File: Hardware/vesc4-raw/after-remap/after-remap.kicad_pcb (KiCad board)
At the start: 4 copper layers, 40.3 x 65 mm, 127 parts, among them K1 SERVO, P1 HALL/Encoder, P101 CANBUS, P2 SWD, P3 PWR_COMM, P4 IN+, P5 IN-, P6 MOTOR1, P7 MOTOR2, P9 MOTOR3, Q1 IPT007N06NATMA1, Q2 IPT007N06NATMA1, Q3 IPT007N06NATMA1, Q4 IPT007N06NATMA1, Q5 IPT007N06NATMA1, Q6 IPT007N06NATMA1, U1 STM32F40X_LQFP64, U2 TC2117, U3 DRV8302, U401 SN65HVD232, X2 8MHz 10ppm

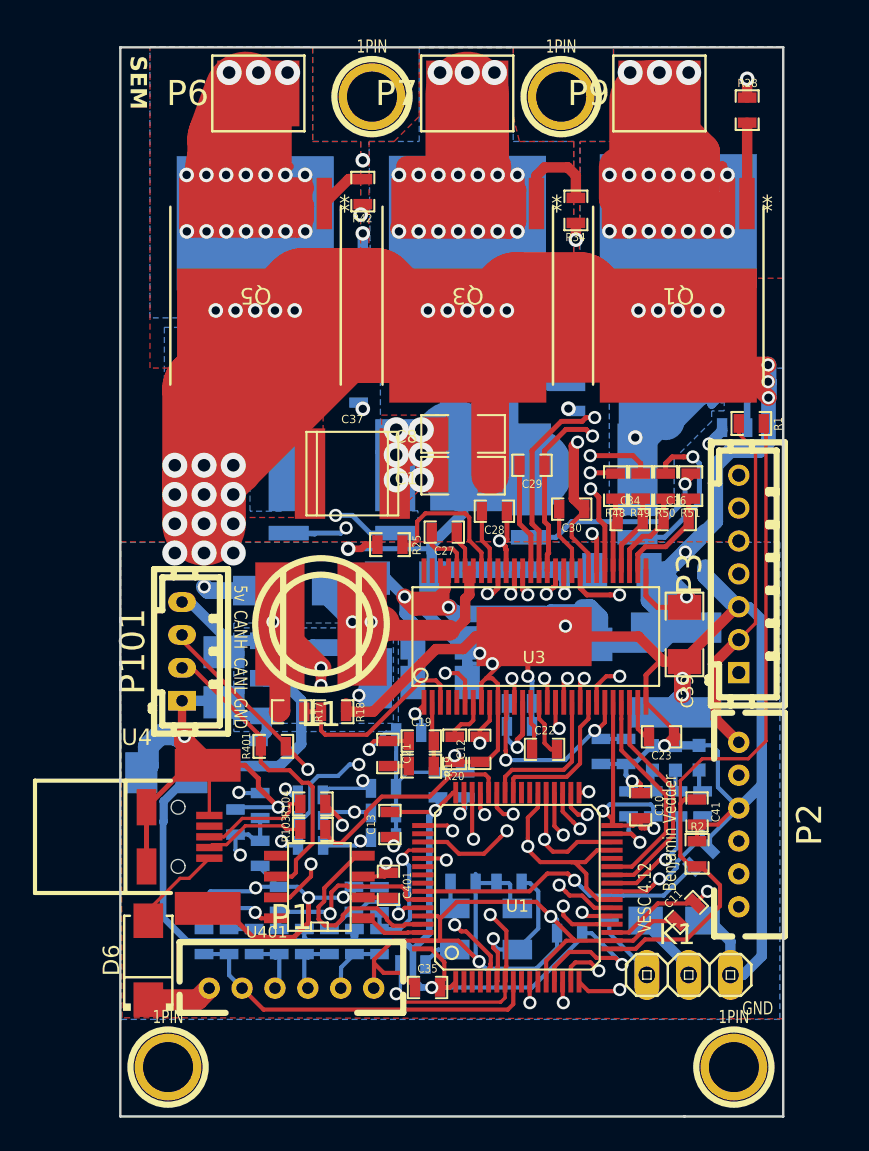
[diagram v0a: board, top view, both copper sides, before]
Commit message: cp
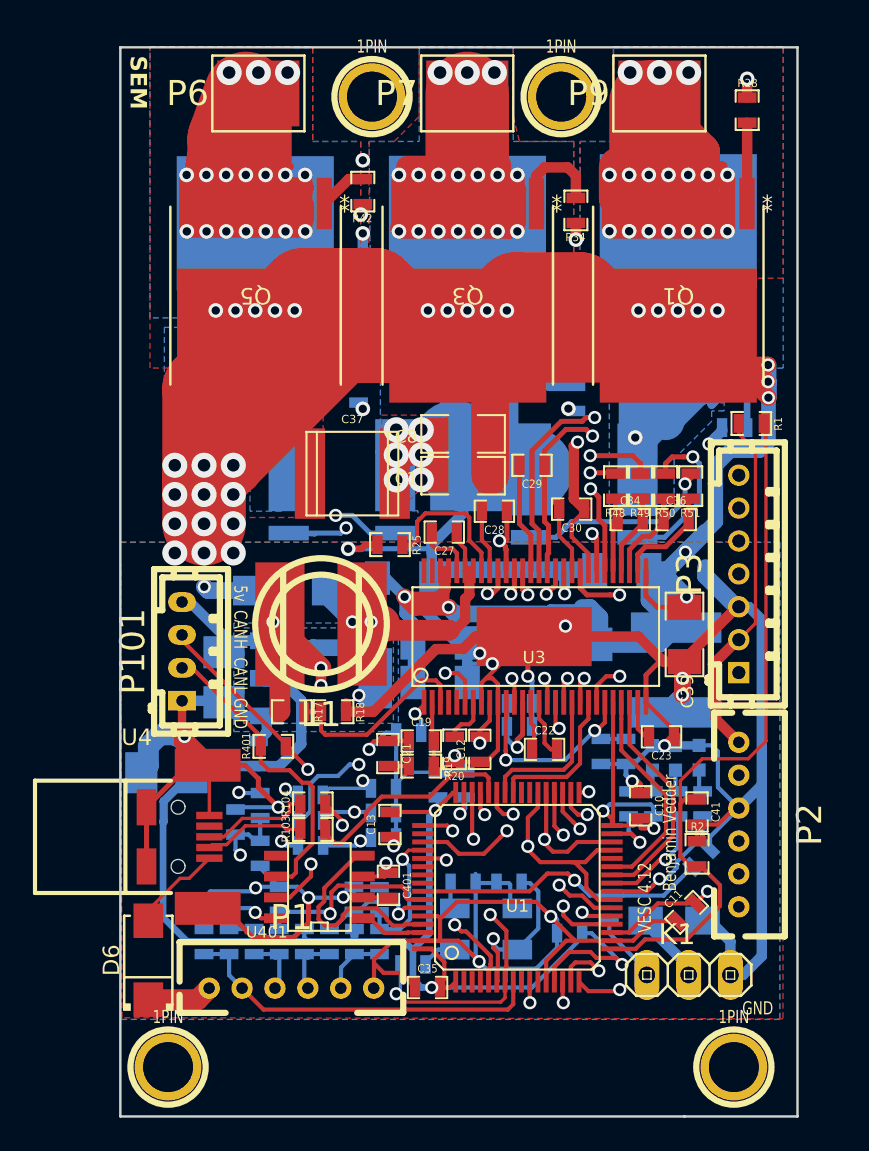
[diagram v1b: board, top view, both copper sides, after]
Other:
- board size 40.3 x 65 mm -> 41.2 x 65 mm
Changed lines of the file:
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@@
 	(gr_line
 		(start 111 145)
-		(end 117 145)
+		(end 117.8681 145)
 		(stroke
 			(width 0.15)
@@
 	)
 	(gr_line
-		(start 117 80)
-		(end 117 145)
+		(start 117.8681 80)
+		(end 117.8681 145)
 		(stroke
 			(width 0.15)
@@
 	)
 	(gr_line
-		(start 117 80)
+		(start 117.8681 80)
 		(end 76.7 80)
 		(stroke
